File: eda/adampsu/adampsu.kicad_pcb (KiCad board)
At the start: 2 copper layers, 121.9 x 58.4 mm, 45 parts, among them J1 Barrel_Jack_Switch, J2 Conn_2Rows-09Pins, J3 DB9_Female, Q1 BUK7880-55A_CUX, SW1 30V 300mA Latching Switch, U1 LM27761, U2 TPS54531DDAR

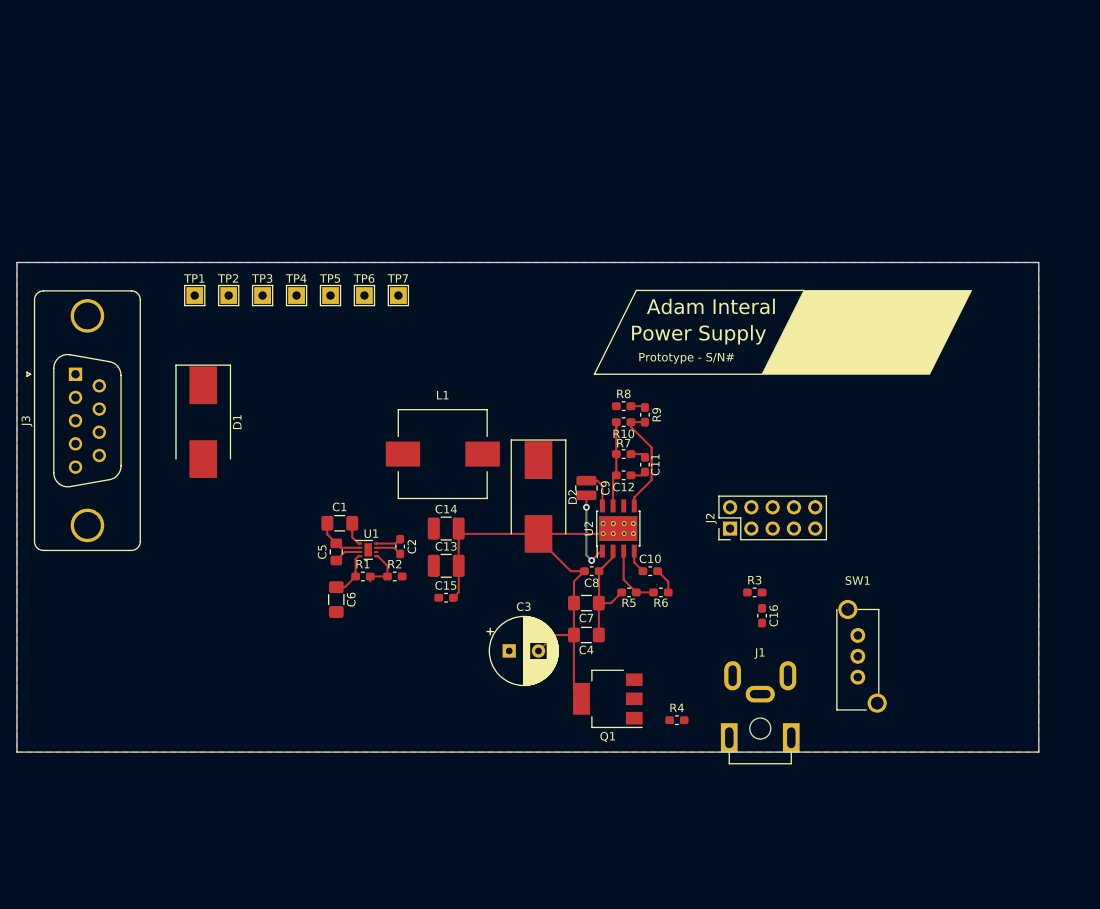
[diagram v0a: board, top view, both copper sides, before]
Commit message: Cleanup
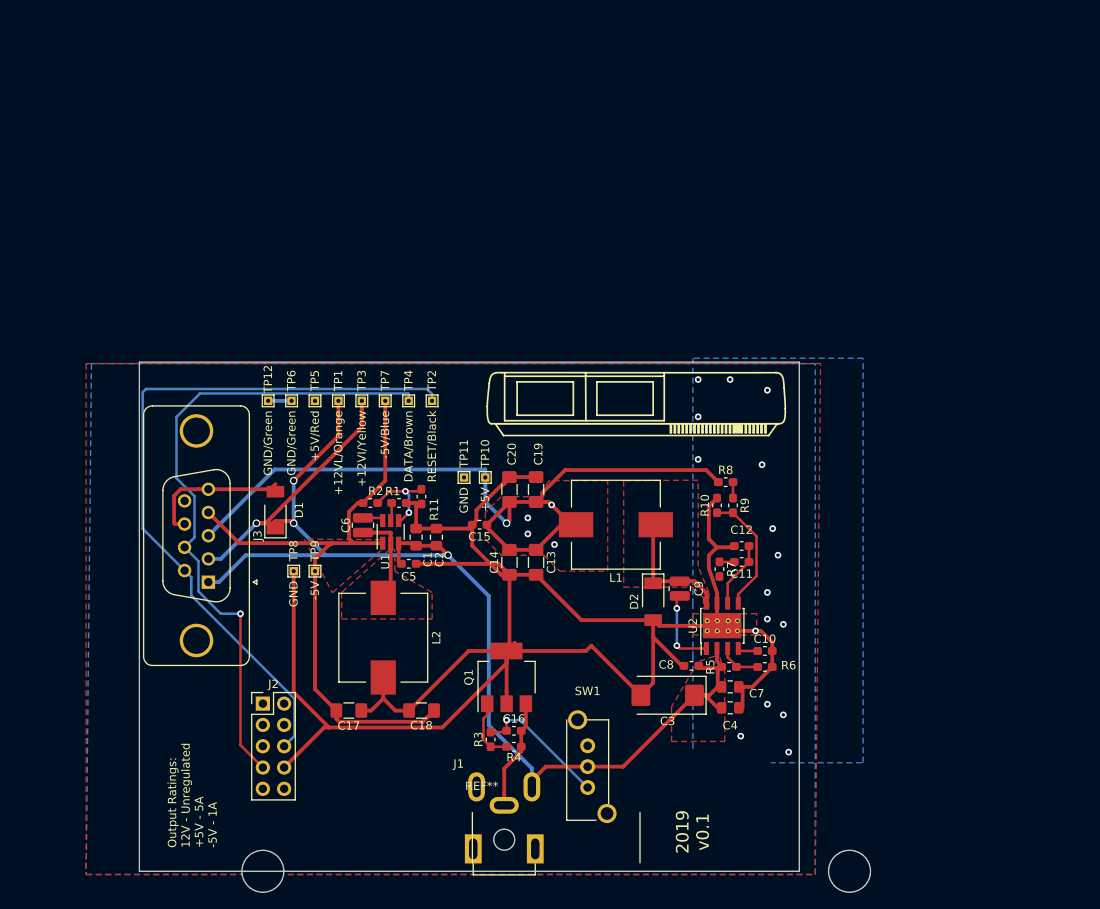
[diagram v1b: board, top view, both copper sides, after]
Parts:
- added C17: 22uF, Capacitor_SMD:C_1206_3216Metric_Pad1.42x1.75mm_HandSolder, F.Cu at (113.3, 139.8)
- added C18: 22uF, Capacitor_SMD:C_1206_3216Metric_Pad1.42x1.75mm_HandSolder, F.Cu at (121.9, 139.8)
- added C19: 22uF, Capacitor_SMD:C_1206_3216Metric_Pad1.42x1.75mm_HandSolder, F.Cu at (135.6, 113.4)
- added C20: 22uF, Capacitor_SMD:C_1206_3216Metric_Pad1.42x1.75mm_HandSolder, F.Cu at (132.4, 113.4)
- added L2: 4.7uH, adampsu:L_11.5x10.3_H4.8, F.Cu at (117.4, 131.1)
- added R11: 54.9k, Resistor_SMD:R_0603_1608Metric_Pad1.05x0.95mm_HandSolder, F.Cu at (121.9, 114.3)
- added REF**: DB9-SpotMount, adampsu:DB9-SpotMount, F.Cu at (138.0, 159.0)
- added TP10: +5V, adampsu:TestPoint_Labeled, F.Cu at (129.5, 112.0)
- added TP11: GND, adampsu:TestPoint_Labeled, F.Cu at (127.0, 112.0)
- added TP12: GND/Green, adampsu:TestPoint_Labeled, F.Cu at (103.6, 102.9)
- added TP8: GND, adampsu:TestPoint_Labeled, F.Cu at (106.7, 123.2)
- added TP9: -5V, adampsu:TestPoint_Labeled, F.Cu at (109.2, 123.2)
- C1: value 4.7uF -> 10uF; footprint Capacitor_SMD:C_1206_3216Metric_Pad1.42x1.75mm_HandSolder -> Capacitor_SMD:C_0805_2012Metric_Pad1.15x1.40mm_HandSolder
- C13, C14: value 47uF -> 22uF; footprint Capacitor_SMD:C_1210_3225Metric_Pad1.42x2.65mm_HandSolder -> Capacitor_SMD:C_1206_3216Metric_Pad1.42x1.75mm_HandSolder
- C2: value 1uF -> 10uF; footprint Capacitor_SMD:C_0603_1608Metric_Pad1.05x0.95mm_HandSolder -> Capacitor_SMD:C_0805_2012Metric_Pad1.15x1.40mm_HandSolder
- C3: footprint Capacitor_THT:CP_Radial_D8.0mm_P3.50mm -> Capacitor_Tantalum_SMD:CP_EIA-7343-43_Kemet-X_Pad2.25x2.55mm_HandSolder
- C4, C7: footprint Capacitor_SMD:C_1206_3216Metric_Pad1.42x1.75mm_HandSolder -> Capacitor_SMD:C_0805_2012Metric_Pad1.15x1.40mm_HandSolder
- C5: value 10uF -> 0.1uF; footprint Capacitor_SMD:C_0805_2012Metric_Pad1.15x1.40mm_HandSolder -> Capacitor_SMD:C_0603_1608Metric_Pad1.05x0.95mm_HandSolder
- C6: value 4.7uF -> 0.1uF; footprint Capacitor_SMD:C_1206_3216Metric_Pad1.42x1.75mm_HandSolder -> adampsu:C_0508_1220Metric_Pad1.40x1.15mm_HandSolder
- D1, D2: footprint Diode_SMD:D_SMC_Handsoldering -> adampsu:D_SOD-128
- LB1: moved to B.Cu
- R1: value 1.55M -> 10k
- R2: value 500k -> 10k
- TP1: value TestPoint -> +12VL/Orange; footprint TestPoint:TestPoint_THTPad_2.0x2.0mm_Drill1.0mm -> adampsu:TestPoint_Labeled
- TP2: value TestPoint -> RESET/Black; footprint TestPoint:TestPoint_THTPad_2.0x2.0mm_Drill1.0mm -> adampsu:TestPoint_Labeled
- TP3: value TestPoint -> +12VI/Yellow; footprint TestPoint:TestPoint_THTPad_2.0x2.0mm_Drill1.0mm -> adampsu:TestPoint_Labeled
- TP4: value TestPoint -> DATA/Brown; footprint TestPoint:TestPoint_THTPad_2.0x2.0mm_Drill1.0mm -> adampsu:TestPoint_Labeled
- TP5: value TestPoint -> +5V/Red; footprint TestPoint:TestPoint_THTPad_2.0x2.0mm_Drill1.0mm -> adampsu:TestPoint_Labeled
- TP6: value TestPoint -> GND/Green; footprint TestPoint:TestPoint_THTPad_2.0x2.0mm_Drill1.0mm -> adampsu:TestPoint_Labeled
- TP7: value TestPoint -> -5V/Blue; footprint TestPoint:TestPoint_THTPad_2.0x2.0mm_Drill1.0mm -> adampsu:TestPoint_Labeled
- U1: value LM27761 -> TPS561201; footprint Package_SON:WSON-8-1EP_2x2mm_P0.5mm_EP0.9x1.6mm -> Package_TO_SOT_SMD:SOT-23-6_Handsoldering
- moved J2 59.5 mm to (103.0, 139.0), turned to 0 degrees
- moved PC1 36.2 mm to (143.5, 166.3)
- moved R3 36.1 mm to (130.2, 143.3), turned to 90 degrees
- moved SW1 34.8 mm to (141.8, 146.5)
- moved J1 33.3 mm to (131.8, 151.1)
- moved C16 32.6 mm to (133.0, 142.2), turned to 0 degrees
- moved J3 29.4 mm to (96.5, 124.5), turned to 270 degrees
- moved TP2 27.3 mm to (123.2, 102.9)
- moved L1 22.3 mm to (145.1, 117.7)
- moved TP1 21.3 mm to (112.0, 102.9)
- moved C7 19.9 mm to (158.8, 137.0), turned to 0 degrees
- moved R4 19.7 mm to (133.0, 144.1)
- moved C3 19.6 mm to (151.3, 138.0), turned to 180 degrees
- moved LB1 19.3 mm to (165.7, 118.7), turned to 270 degrees
- moved C4 19.2 mm to (158.8, 139.5), turned to 0 degrees
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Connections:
- net Net-(C9-Pad1) renamed /PH
- C1 pad 1: +5V -> +12V
- C14 pad 1: +5V -> GND
- C14 pad 2: GND -> +5V
- C2 pad 1: Net-(C2-Pad1) -> +12V
- C2 pad 2: Net-(C2-Pad2) -> GND
- C5 pad 1: Net-(C5-Pad1) -> +12V
- C6 pad 2: GND -> /SW
- D1 pad 1: /+12VI -> +12V
- J3 pad 1: /+12VL -> +12V
- J3 pad 2: /+12VI -> +12V
- R1 pad 1: Net-(C6-Pad1) -> GND
- R2 pad 1: Net-(R1-Pad2) -> /-5V
- R2 pad 2: GND -> Net-(R11-Pad2)
- TP1 pad 1: /+12VL -> +12V
- TP3 pad 1: /+12VI -> +12V
- U1 pad 1: +5V -> /-5V
- U1 pad 2: GND -> /SW
- U1 pad 3: Net-(C5-Pad1) -> +12V
- U1 pad 4: Net-(C6-Pad1) -> Net-(R11-Pad2)
- U1 pad 6: Net-(U1-Pad6) -> Net-(C6-Pad1)
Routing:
- net GND: track 76.1 -> 253.2 mm, vias 0 -> 16
- net +12V: track 13.9 -> 164.4 mm, vias 0 -> 4
- net +5V: track 2.94 -> 96.8 mm, vias 0 -> 5
- net /RESET: track 0.00 -> 86.0 mm
- net /DATA: track 0.00 -> 78.1 mm, vias 0 -> 1
- net /-5V: track 0.00 -> 77.2 mm
- net Net-(C16-Pad1): track 0.00 -> 16.4 mm, vias 0 -> 1
- net /GND-F: track 0.00 -> 13.2 mm
- net /SW: track 0.00 -> 11.5 mm
- net /PH: track 4.57 -> 15.4 mm
- net Net-(R11-Pad2): track 0.00 -> 10.2 mm, vias 0 -> 2
- net Net-(Q1-Pad1): track 0.00 -> 7.58 mm
- net Net-(C11-Pad1): track 1.83 -> 7.88 mm
- net Net-(C5-Pad1): track 3.28 -> 0.00 mm
- net Net-(C2-Pad2): track 3.16 -> 0.00 mm
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- added copper zone on F.Cu, net +12V
- added copper zone on B.Cu, net +5V
- added copper zone on F.Cu, net +5V
- added copper zone on F.Cu, net /-5V
- added copper zone on F.Cu, net /PH
- added copper zone on F.Cu, net /SW
- added copper zone on B.Cu, net GND
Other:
- board size 121.9 x 58.4 mm -> 78.7 x 60.8 mm
- net class Default: clearance 0.2 -> 0.2286; trace_width 0.25 -> 0.3048
- net class Power added: clearance 0.2286, trace_width 0.4572, via_dia 0.9144, via_drill 0.6096
- rule trace_clearance: 0.2 -> 0.2286
- board text added: "2019 v0.1"
- board text added: "By Shelby Jueden"
- board text added: "Output Ratings: 12V - Unregulated +5V - 5A -5V - 1A"
- board text added: "https://github.com/AkBKukU/adam-psu"

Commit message: Export schematic and PCB to PDFs
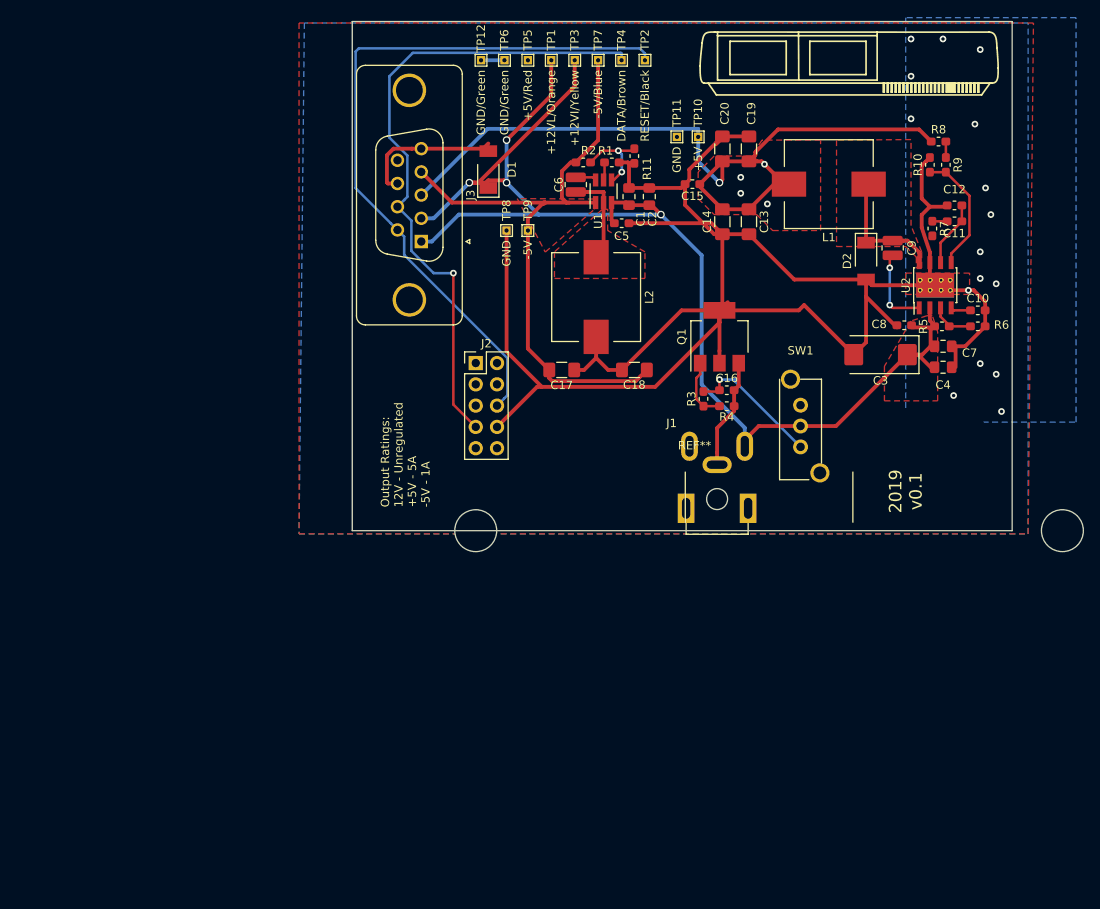
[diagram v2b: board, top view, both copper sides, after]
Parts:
- moved C17 47.9 mm to (138.7, 99.2)
- moved C18 47.9 mm to (147.3, 99.2)
- moved SW1 47.9 mm to (167.2, 105.9)
- moved C1 47.9 mm to (146.7, 78.5)
- moved C10 47.9 mm to (188.3, 92.1)
- moved C11 47.9 mm to (185.5, 81.5)
- moved C12 47.9 mm to (185.5, 79.5)
- moved C13 47.9 mm to (161.0, 81.5)
- moved C15 47.9 mm to (154.3, 77.0)
- moved C19 47.9 mm to (161.0, 72.8)
- moved C2 47.9 mm to (149.1, 78.5)
- moved C4 47.9 mm to (184.2, 98.9)
- moved C6 47.9 mm to (140.3, 77.1)
- moved C7 47.9 mm to (184.2, 96.4)
- moved C8 47.9 mm to (179.5, 93.9)
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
